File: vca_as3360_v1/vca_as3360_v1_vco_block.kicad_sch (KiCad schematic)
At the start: 6 parts, among them U1 AS3360

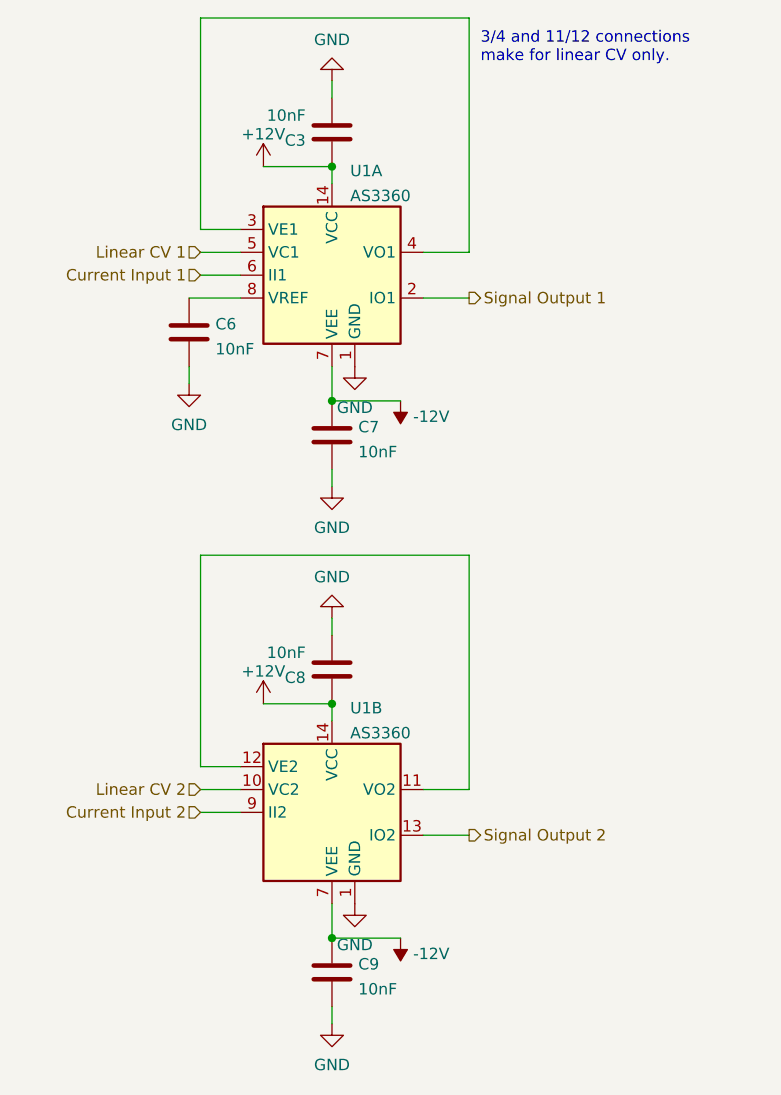
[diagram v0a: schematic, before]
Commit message: Layout and routing first pass done
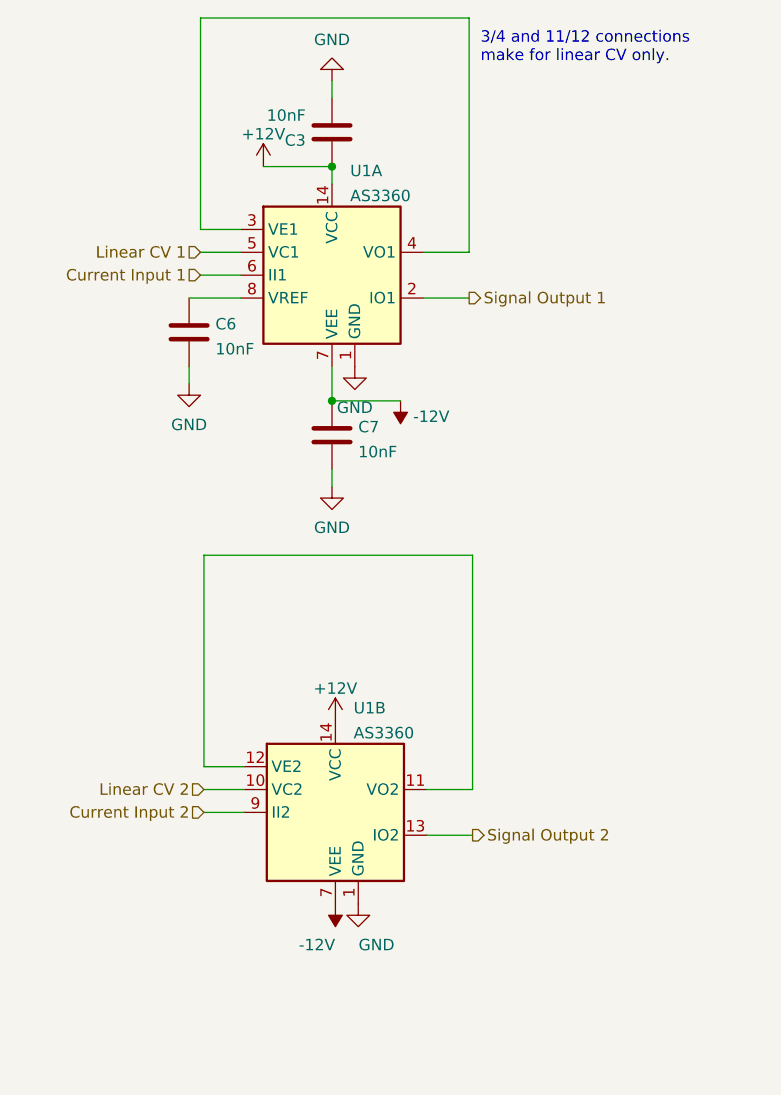
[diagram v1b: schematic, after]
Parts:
- removed C8, C9: 10nF, Capacitor_SMD:C_1206_3216Metric_Pad1.33x1.80mm_HandSolder, symbol Device:C
